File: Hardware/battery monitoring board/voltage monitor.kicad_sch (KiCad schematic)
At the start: 14 parts, among them J1 S5B-XH-A

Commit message: Added footprints to battery monitoring
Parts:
- C1, C2, C3: footprint (none) -> Capacitor_SMD:C_0805_2012Metric_Pad1.18x1.45mm_HandSolder
- J1: footprint S5B-XH-A:JST_S5B-XH-A -> Library:JST_S5B-XH-A
- R1, R2, R3, R4, R5, R6, R7: footprint (none) -> Resistor_SMD:R_0805_2012Metric_Pad1.20x1.40mm_HandSolder
- TP1: footprint (none) -> Library:Test Pads
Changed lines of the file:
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@@
       (effects (font (size 1.27 1.27)) (justify left))
     )
-    (property "Footprint" "" (at 37.846 39.624 90)
+    (property "Footprint" "Resistor_SMD:R_0805_2012Metric_Pad1.20x1.40mm_HandSolder" (at 37.846 39.624 90)
       (effects (font (size 1.27 1.27)) hide)
     )
@@
       (effects (font (size 1.27 1.27)) (justify right))
     )
-    (property "Footprint" "" (at 48.514 39.116 90)
+    (property "Footprint" "Resistor_SMD:R_0805_2012Metric_Pad1.20x1.40mm_HandSolder" (at 48.514 39.116 90)
       (effects (font (size 1.27 1.27)) hide)
     )
@@
       (effects (font (size 1.27 1.27)) (justify left))
     )
-    (property "Footprint" "" (at 120.3452 43.18 0)
+    (property "Footprint" "Capacitor_SMD:C_0805_2012Metric_Pad1.18x1.45mm_HandSolder" (at 120.3452 43.18 0)
       (effects (font (size 1.27 1.27)) hide)
     )
@@
       (effects (font (size 1.27 1.27)) (justify left))
     )
-    (property "Footprint" "" (at 61.9252 43.18 0)
+    (property "Footprint" "Capacitor_SMD:C_0805_2012Metric_Pad1.18x1.45mm_HandSolder" (at 61.9252 43.18 0)
       (effects (font (size 1.27 1.27)) hide)
     )
@@
       (effects (font (size 1.27 1.27)) (justify left))
     )
-    (property "Footprint" "" (at 79.756 39.624 90)
+    (property "Footprint" "Resistor_SMD:R_0805_2012Metric_Pad1.20x1.40mm_HandSolder" (at 79.756 39.624 90)
       (effects (font (size 1.27 1.27)) hide)
     )
@@
       (effects (font (size 1.27 1.27)) (justify left))
     )
-    (property "Footprint" "" (at 124.46 35.56 0)
+    (property "Footprint" "Library:Test Pads" (at 124.46 35.56 0)
       (effects (font (size 1.27 1.27)) hide)
     )
@@
       (effects (font (size 1.27 1.27)) (justify right))
     )
-    (property "Footprint" "" (at 77.724 27.178 90)
+    (property "Footprint" "Resistor_SMD:R_0805_2012Metric_Pad1.20x1.40mm_HandSolder" (at 77.724 27.178 90)
       (effects (font (size 1.27 1.27)) hide)
     )
@@
       (effects (font (size 1.27 1.27)) (justify right))
     )
-    (property "Footprint" "" (at 48.514 27.432 90)
+    (property "Footprint" "Resistor_SMD:R_0805_2012Metric_Pad1.20x1.40mm_HandSolder" (at 48.514 27.432 90)
       (effects (font (size 1.27 1.27)) hide)
     )
@@
       (effects (font (size 1.27 1.27)) (justify left))
     )
-    (property "Footprint" "" (at 108.966 39.624 90)
+    (property "Footprint" "Resistor_SMD:R_0805_2012Metric_Pad1.20x1.40mm_HandSolder" (at 108.966 39.624 90)
       (effects (font (size 1.27 1.27)) hide)
     )
@@
       (effects (font (size 1.27 1.27)) (justify left))
     )
-    (property "Footprint" "" (at 91.1352 43.18 0)
+    (property "Footprint" "Capacitor_SMD:C_0805_2012Metric_Pad1.18x1.45mm_HandSolder" (at 91.1352 43.18 0)
       (effects (font (size 1.27 1.27)) hide)
     )
@@
       (effects (font (size 1.27 1.27)) (justify right))
     )
-    (property "Footprint" "" (at 106.934 27.686 90)
+    (property "Footprint" "Resistor_SMD:R_0805_2012Metric_Pad1.20x1.40mm_HandSolder" (at 106.934 27.686 90)
       (effects (font (size 1.27 1.27)) hide)
     )
@@
       (effects (font (size 1.27 1.27)))
     )
-    (property "Footprint" "S5B-XH-A:JST_S5B-XH-A" (at 26.67 31.75 0)
+    (property "Footprint" "Library:JST_S5B-XH-A" (at 26.67 31.75 0)
       (effects (font (size 1.27 1.27)) (justify bottom) hide)
     )
@@
       (effects (font (size 1.27 1.27)) (justify left))
     )
-    (property "Footprint" "" (at 66.04 35.56 0)
+    (property "Footprint" "Library:Test Pads" (at 66.04 35.56 0)
       (effects (font (size 1.27 1.27)) hide)
     )
@@
       (effects (font (size 1.27 1.27)) (justify left))
     )
-    (property "Footprint" "" (at 95.25 35.56 0)
-      (effects (font (size 1.27 1.27)) hide)
-    )
+    (property "Footprint" "Library:Test Pads" (at 95.25 35.56 0)
+      (effects (font (size 1.27 1.27)) hide)
+    )

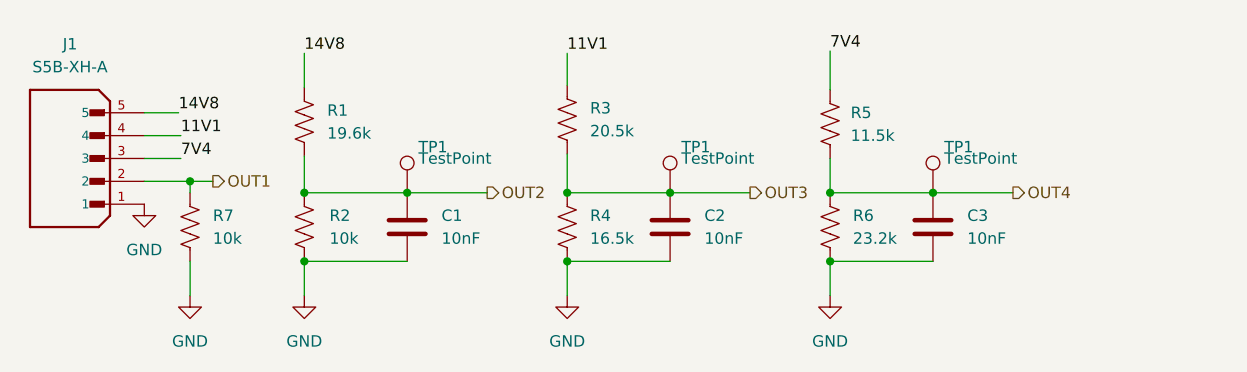
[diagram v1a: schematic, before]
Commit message: Added adc to schematic
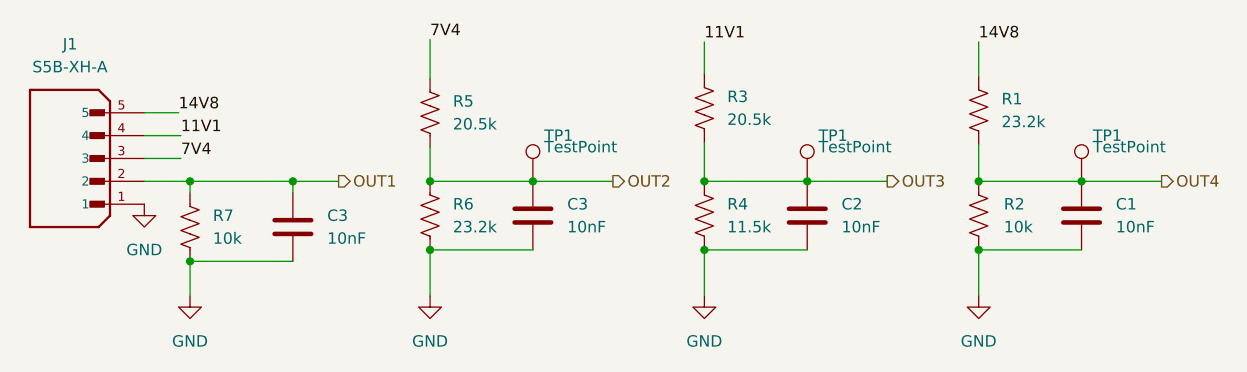
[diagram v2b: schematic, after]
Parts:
- added C3: 10nF, Capacitor_SMD:C_0805_2012Metric_Pad1.18x1.45mm_HandSolder, symbol Device:C
- R1: value 19.6k -> 23.2k
- R4: value 16.5k -> 11.5k
- R5: value 11.5k -> 20.5k
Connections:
- net GND: now also C3.2
- net OUT1: now also C3.1
- net OUT2: now also C3.1, R5.1, R6.1, TP1.1; no longer C1.1, R1.1, R2.2, TP1.1
- net OUT4: now also C1.1, R1.1, R2.2, TP1.1; no longer C3.1, R5.1, R6.1, TP1.1
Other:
- moved on the sheet: C1, C2, C3, R1, R2, R3, R4, R5, R6, TP1
